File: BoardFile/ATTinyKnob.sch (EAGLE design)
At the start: 16 parts, among them U1 ATTINY_25_45_85

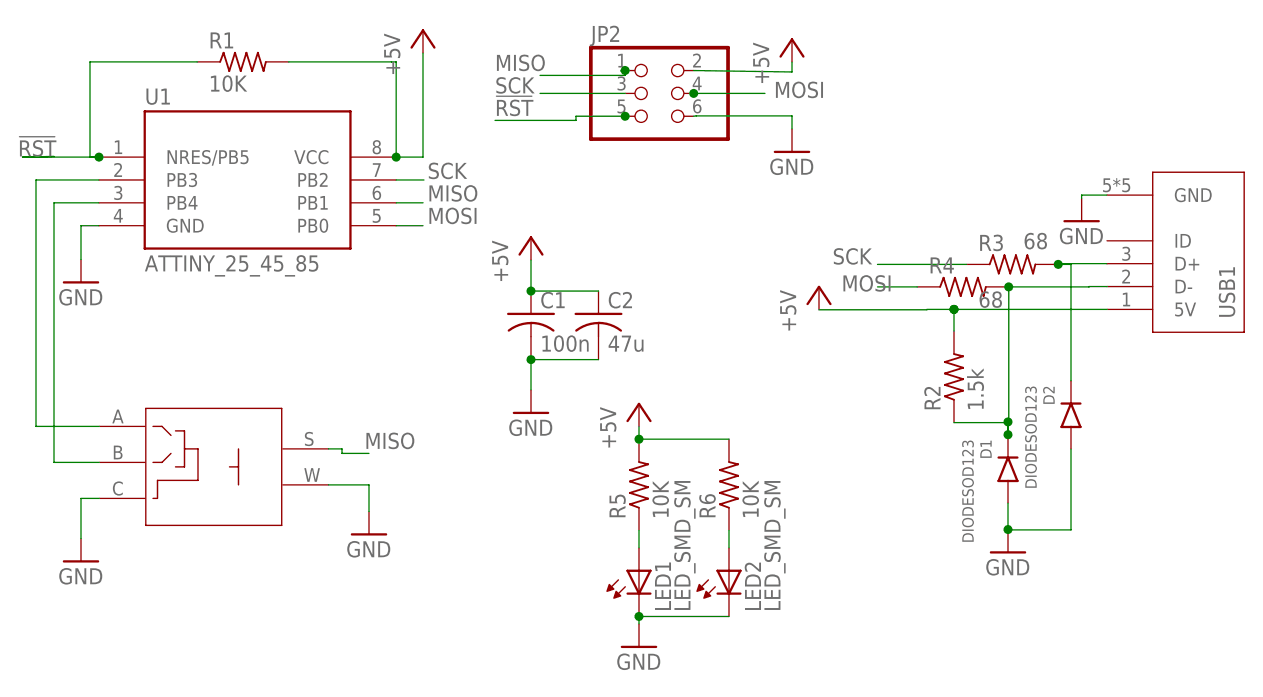
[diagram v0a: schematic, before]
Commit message: Board built
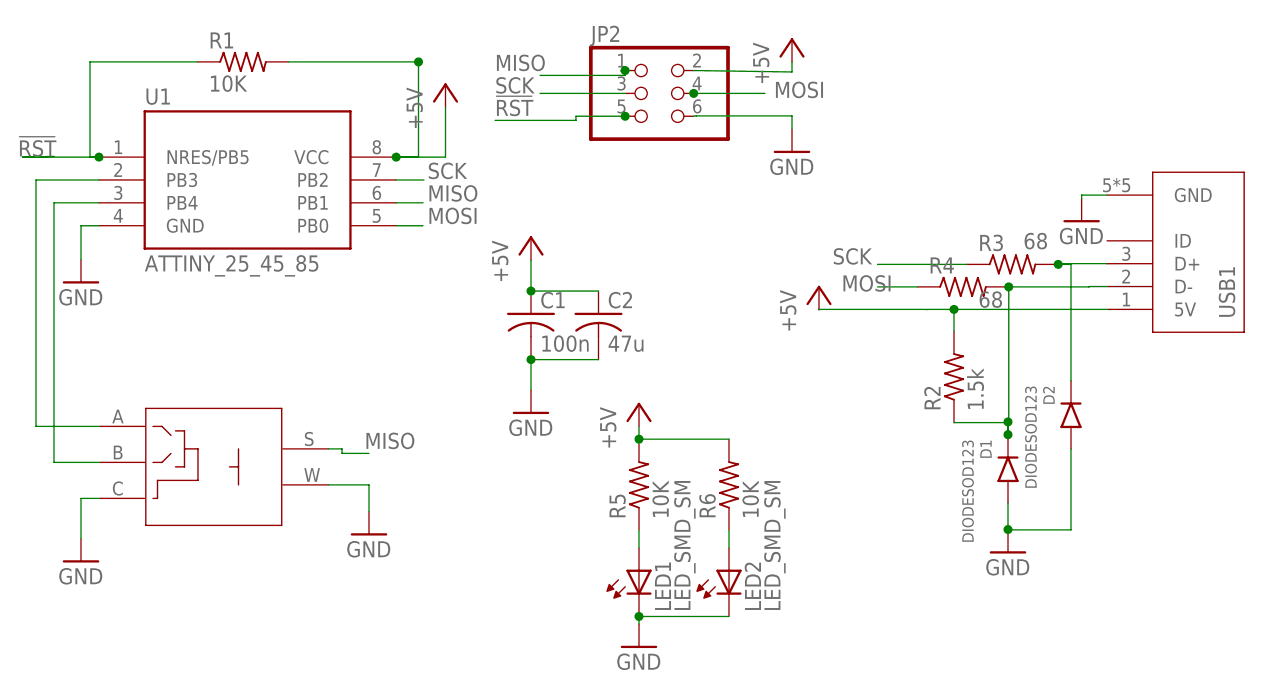
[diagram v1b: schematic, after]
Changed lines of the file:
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@@
 <attribute name="VALUE" x="126.64" y="100.26" size="1.778" layer="96"/>
 </instance>
-<instance part="P+1" gate="1" x="56" y="124" smashed="yes">
-<attribute name="VALUE" x="53.46" y="118.92" size="1.778" layer="96" rot="R90"/>
+<instance part="P+1" gate="1" x="58.5" y="118" smashed="yes">
+<attribute name="VALUE" x="55.96" y="112.92" size="1.778" layer="96" rot="R90"/>
 </instance>
 <instance part="ROT1" gate="G$1" x="20" y="80" smashed="yes">
@@
 <net name="+5V" class="0">
 <segment>
+<pinref part="P+1" gate="1" pin="+5V"/>
+<wire x1="58.5" y1="109.92" x2="58.5" y2="115.46" width="0.1524" layer="91"/>
 <pinref part="U1" gate="G$1" pin="VCC"/>
-<pinref part="P+1" gate="1" pin="+5V"/>
-<wire x1="53.02" y1="109.92" x2="56" y2="109.92" width="0.1524" layer="91"/>
-<wire x1="56" y1="109.92" x2="56" y2="121.46" width="0.1524" layer="91"/>
+<wire x1="53.02" y1="109.92" x2="58.5" y2="109.92" width="0.1524" layer="91"/>
 <pinref part="R1" gate="G$1" pin="2"/>
-<wire x1="41.08" y1="120.5" x2="52.5" y2="120.5" width="0.1524" layer="91"/>
-<wire x1="52.5" y1="120.5" x2="53.02" y2="120.5" width="0.1524" layer="91"/>
-<wire x1="53.02" y1="120.5" x2="53.02" y2="109.92" width="0.1524" layer="91"/>
+<wire x1="41.08" y1="120.5" x2="55.5" y2="120.5" width="0.1524" layer="91"/>
+<wire x1="55.5" y1="120.5" x2="55.52" y2="120.5" width="0.1524" layer="91"/>
+<wire x1="55.5" y1="120.5" x2="55.5" y2="109.92" width="0.1524" layer="91"/>
+<wire x1="55.5" y1="109.92" x2="53.02" y2="109.92" width="0.1524" layer="91"/>
+<junction x="55.5" y="120.5"/>
 <junction x="53.02" y="109.92"/>
 </segment>
@@
 </segment>
 <segment>
+<pinref part="P+2" gate="1" pin="+5V"/>
+<pinref part="USB1" gate="G$1" pin="5V"/>
+<pinref part="R2" gate="G$1" pin="2"/>
 <wire x1="132" y1="93" x2="115" y2="93" width="0.1524" layer="91"/>
-<pinref part="P+2" gate="1" pin="+5V"/>
-<wire x1="115" y1="93" x2="112" y2="93" width="0.1524" layer="91"/>
-<wire x1="112" y1="93" x2="112" y2="92.96" width="0.1524" layer="91"/>
-<wire x1="112" y1="92.96" x2="100" y2="92.96" width="0.1524" layer="91"/>
-<pinref part="R2" gate="G$1" pin="2"/>
-<wire x1="115" y1="90.58" x2="115" y2="93" width="0.1524" layer="91"/>
+<wire x1="115" y1="93" x2="115" y2="90.58" width="0.1524" layer="91"/>
+<wire x1="115" y1="93" x2="100" y2="93" width="0.1524" layer="91"/>
+<wire x1="100" y1="93" x2="100" y2="92.96" width="0.1524" layer="91"/>
 <junction x="115" y="93"/>
-<pinref part="USB1" gate="G$1" pin="5V"/>
 </segment>
 <segment>
@@
 </segment>
 </net>
-<net name="N$3" class="0">
-<segment>
-<junction x="115" y="93"/>
-</segment>
-</net>
 <net name="N$7" class="0">
 <segment>
@@
 </segment>
 </net>
+<net name="N$5" class="0">
+<segment>
+<wire x1="112" y1="93" x2="112" y2="92.96" width="0.1524" layer="91"/>
+</segment>
+</net>
 </nets>
 </sheet>
 </sheets>
-<errors>
-</errors>
 </schematic>
 </drawing>
